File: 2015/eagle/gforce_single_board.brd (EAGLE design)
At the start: 64.4 x 59.7 mm, 28 parts, among them U1 ATMEGA328P_PDIP

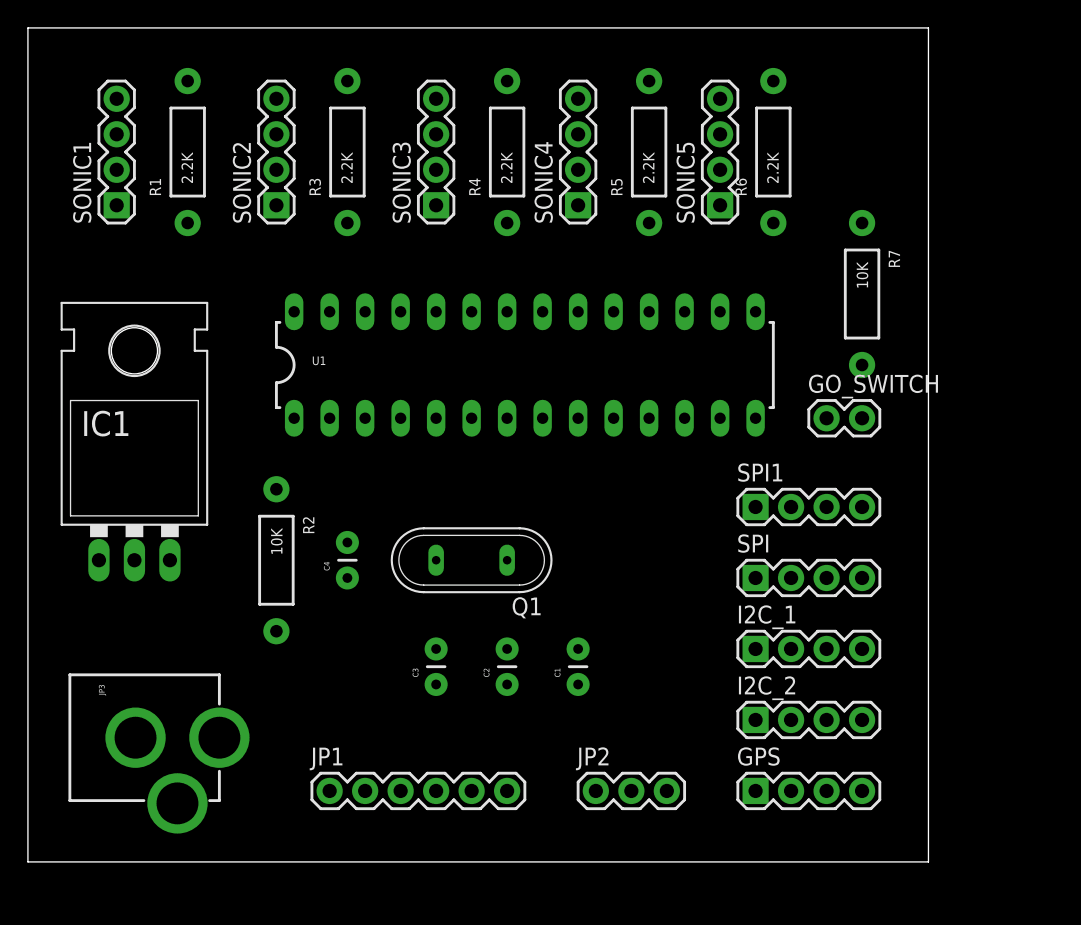
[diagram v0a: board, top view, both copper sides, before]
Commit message: save
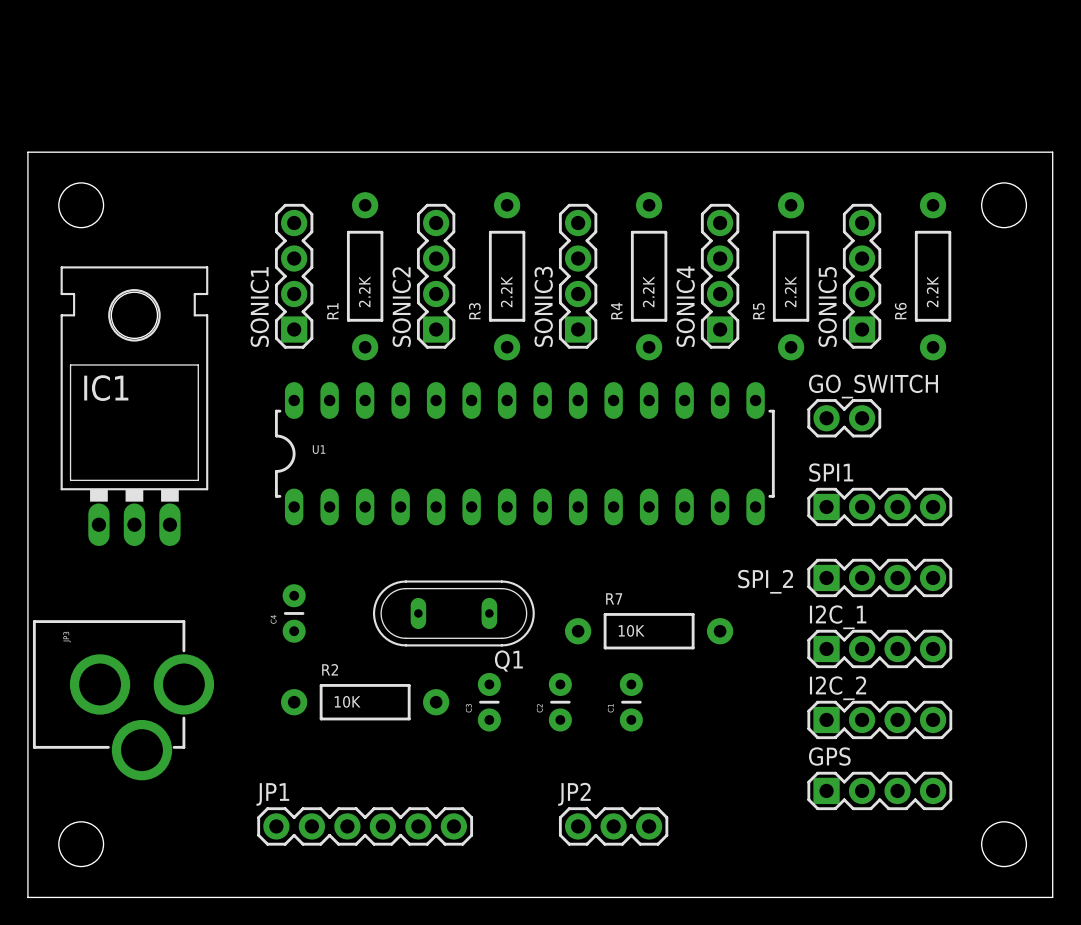
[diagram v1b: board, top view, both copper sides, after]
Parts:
- removed SPI: (no value), SparkFun-Connectors:1X04
- added SPI_2: (no value), SparkFun-Connectors:1X04
- moved R7 28.5 mm to (44.5, 16.5), turned to 0 degrees
- moved SONIC1 15.5 mm to (19.1, 38.1)
- moved R1 15.5 mm to (24.1, 41.9)
- moved R3 14.5 mm to (34.3, 41.9)
- moved SONIC2 14.5 mm to (29.2, 38.1)
- moved R6 14.5 mm to (64.8, 41.9)
- moved R4 13.5 mm to (44.5, 41.9)
- moved SONIC4 13.5 mm to (49.5, 38.1)
- moved R5 13.5 mm to (54.6, 41.9)
- moved SONIC3 13.5 mm to (39.4, 38.1)
- moved SONIC5 13.5 mm to (59.7, 38.1)
- moved R2 12.0 mm to (24.1, 11.4), turned to 0 degrees
- moved U1 6.35 mm to (35.6, 29.2)
- moved C4 5.39 mm to (19.1, 16.5)
- moved GPS 5.08 mm to (57.1, 5.08)
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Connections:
- net MISO: now also SPI_2.2; no longer SPI.2
- net MOSI: now also SPI_2.3; no longer SPI.3
- net N$22: now also SPI_2.4; no longer SPI.4
- net SCK: now also SPI_2.1; no longer SPI.1
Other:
- board size 64.4 x 59.7 mm -> 73.3 x 53.3 mm
